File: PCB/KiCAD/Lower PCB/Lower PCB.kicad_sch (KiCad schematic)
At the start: 16 parts, among them J2 Conn_01x02, U1 ATmega328PB-A, Y1 Crystal

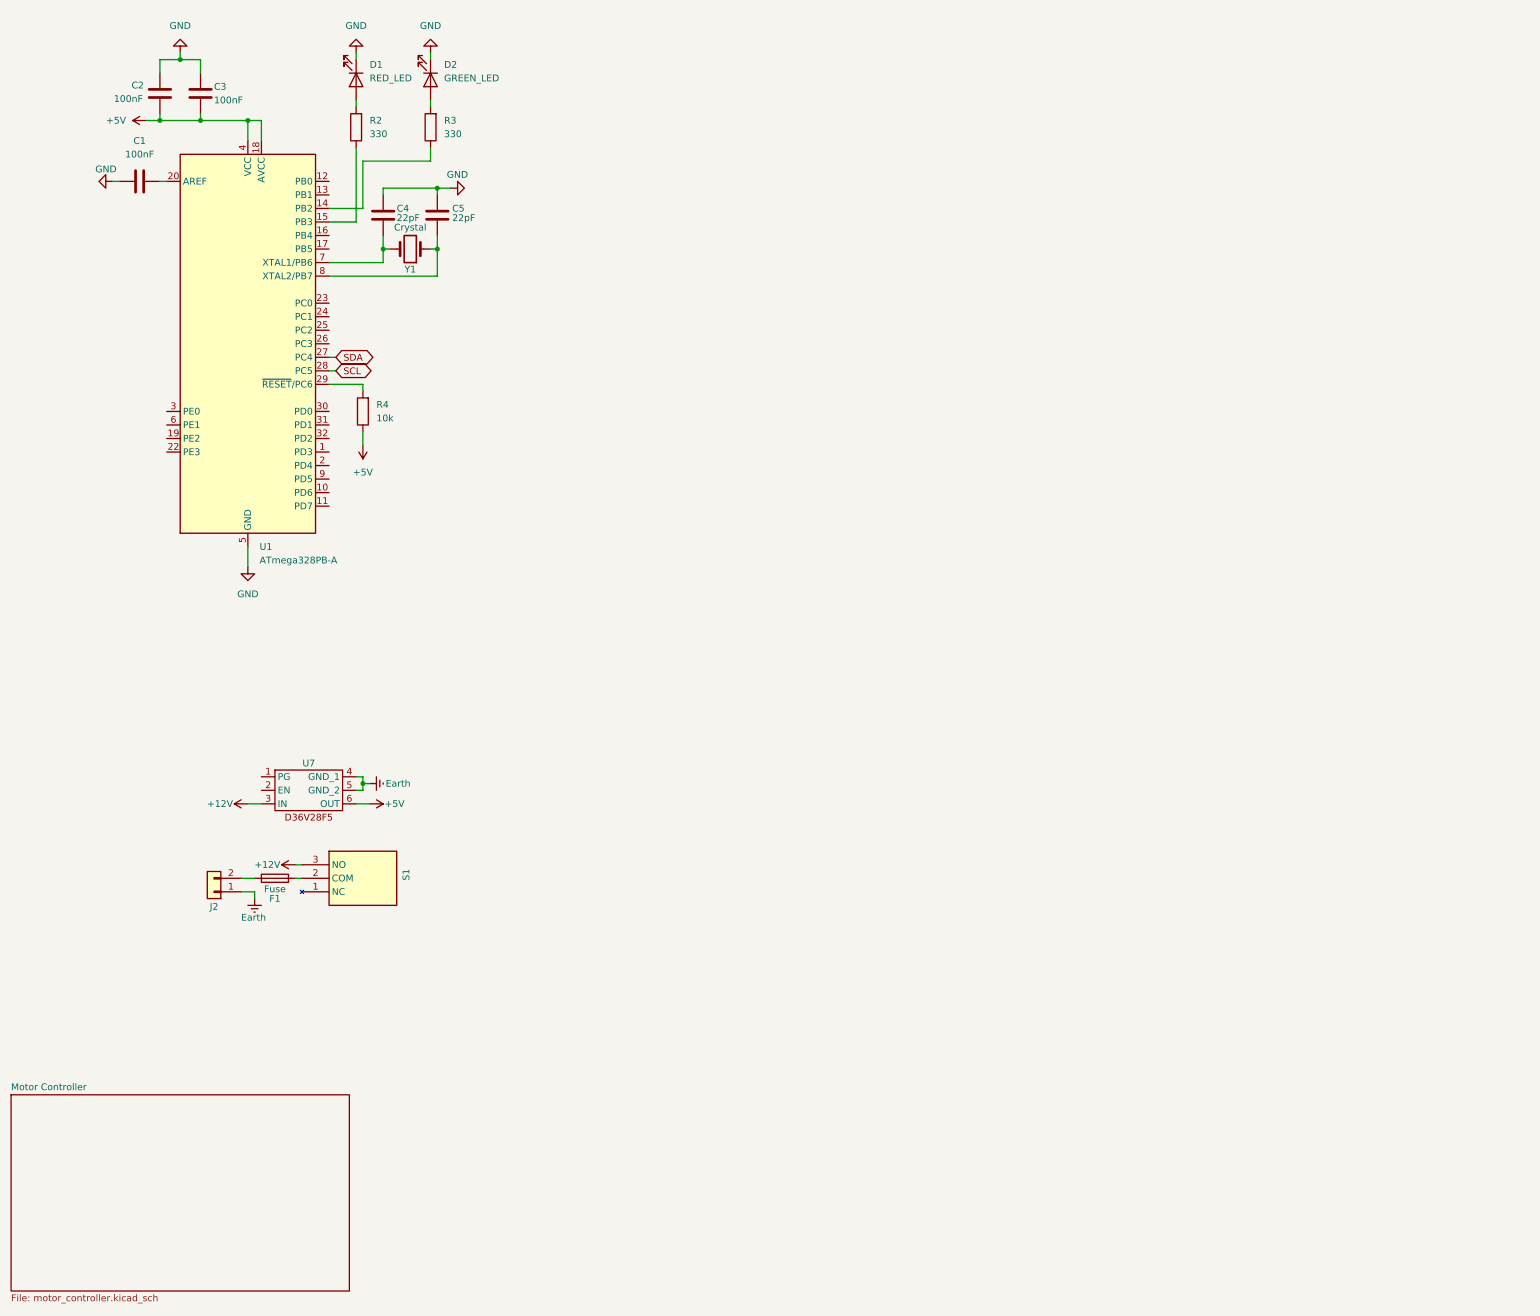
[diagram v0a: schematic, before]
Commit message: More work to the lower PCB
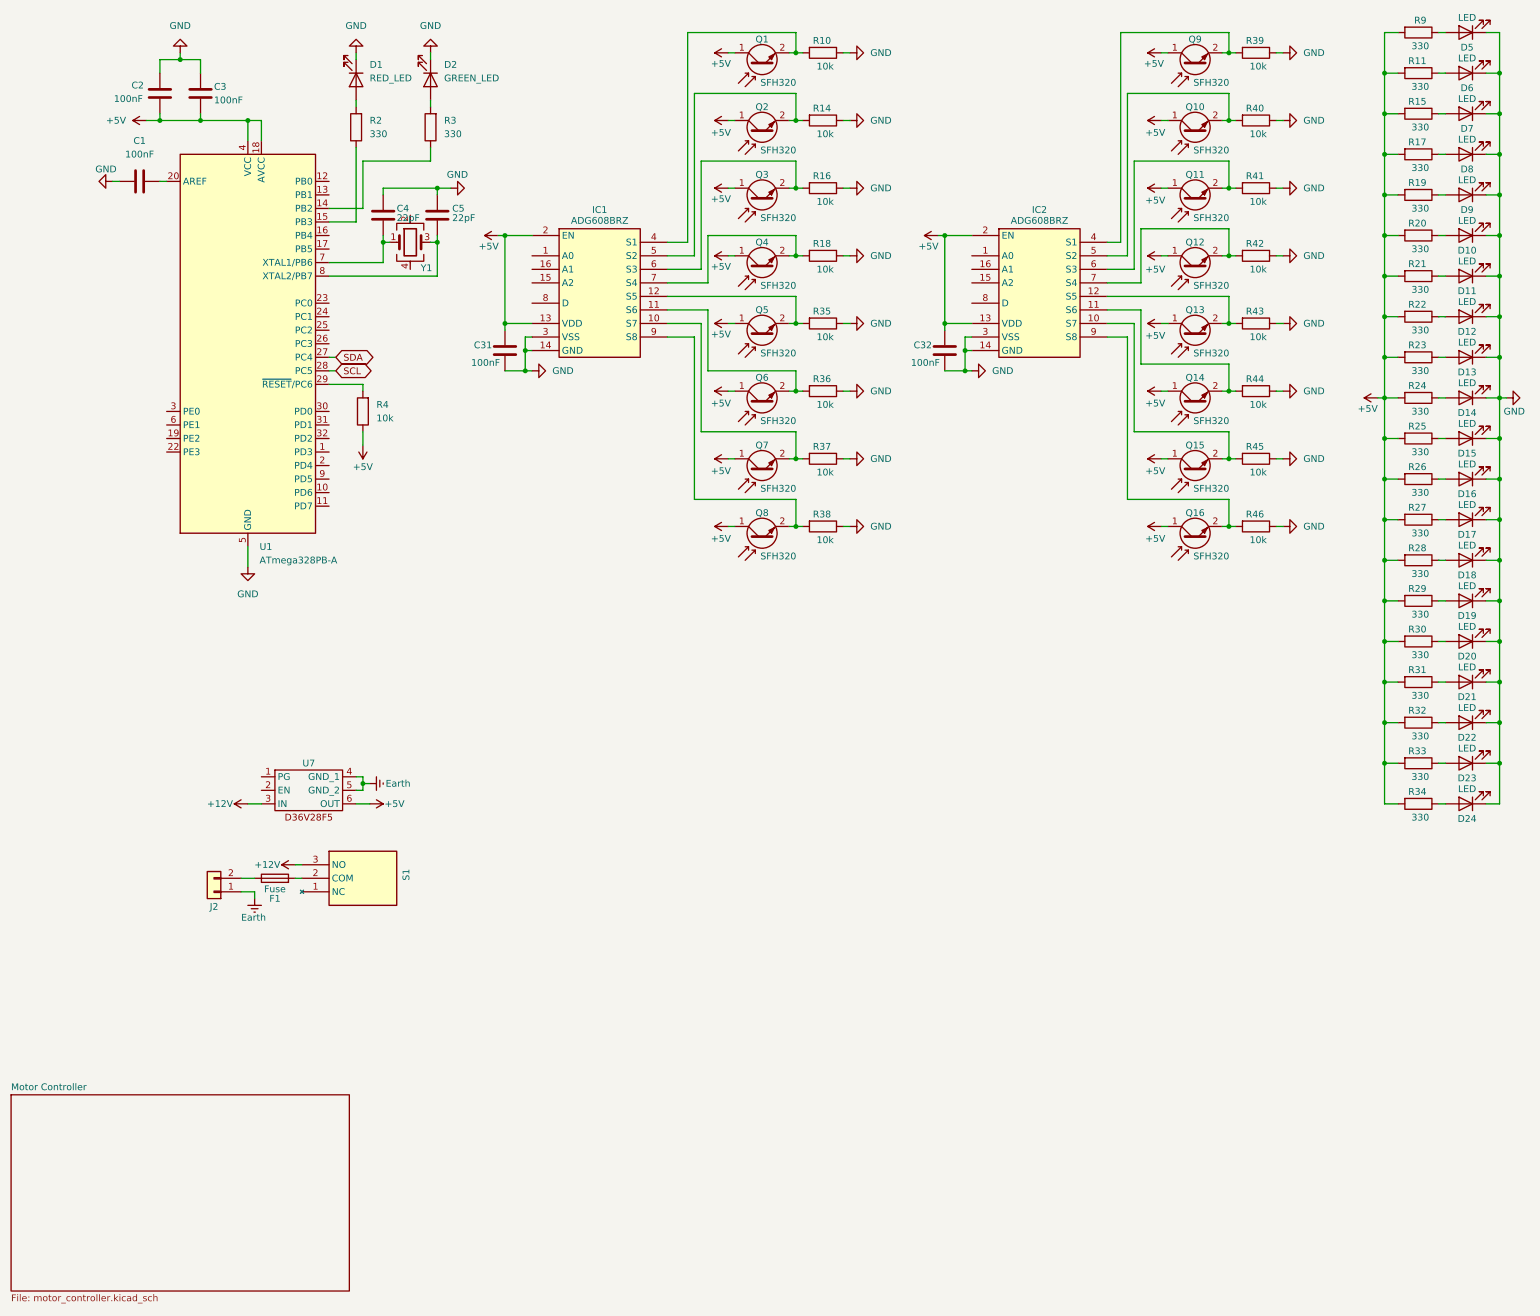
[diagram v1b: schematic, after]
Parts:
- removed Y1: Crystal, Crystal:Crystal_SMD_3225-4Pin_3.2x2.5mm_HandSoldering, symbol Device:Crystal
- added C31, C32: 100nF, Capacitor_SMD:C_0805_2012Metric_Pad1.18x1.45mm_HandSolder, symbol Device:C
- added D10, D11, D12, D13, D14, D15, D16, D17, D18, D19, D20, D21, D22, D23, D24, D5, D6, D7, D8, D9: LED, LED_SMD:LED_PLCC-2_3.4x3.0mm_KA, symbol Device:LED
- added IC1, IC2: ADG608BRZ, ADG608BRZ:SOIC127P600X175-16N, symbol ADG608BRZ:ADG608BRZ
- added Q1, Q10, Q11, Q12, Q13, Q14, Q15, Q16, Q2, Q3, Q4, Q5, Q6, Q7, Q8, Q9: SFH320, LED_SMD:LED_PLCC-2_3.4x3.0mm_KA, symbol Sensor_Optical:SFH320
- added R10, R14, R16, R18, R35, R36, R37, R38, R39, R40, R41, R42, R43, R44, R45, R46: 10k, Resistor_SMD:R_0805_2012Metric_Pad1.20x1.40mm_HandSolder, symbol Device:R
- added R11, R15, R17, R19, R20, R21, R22, R23, R24, R25, R26, R27, R28, R29, R30, R31, R32, R33, R34, R9: 330, Resistor_SMD:R_0805_2012Metric_Pad1.20x1.40mm_HandSolder, symbol Device:R
- added Y1: Crystal_GND24, Crystal:Crystal_SMD_5032-4Pin_5.0x3.2mm, symbol Device:Crystal_GND24
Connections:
- net +5V: now also C31.1, C32.1, IC1.13 (VDD), IC1.2 (EN), IC2.13 (VDD), IC2.2 (EN), Q1.1 (C), Q10.1 (C), Q11.1 (C), Q12.1 (C), Q13.1 (C), Q14.1 (C), Q15.1 (C), Q16.1 (C), Q2.1 (C), Q3.1 (C), Q4.1 (C), Q5.1 (C), Q6.1 (C), Q7.1 (C), Q8.1 (C), Q9.1 (C), R11.2, R15.2, R17.2, R19.2, R20.2, R21.2, R22.2, R23.2, R24.2, R25.2, R26.2, R27.2, R28.2, R29.2, R30.2, R31.2, R32.2, R33.2, R34.2, R9.2
- net GND: now also C31.2, C32.2, D10.1 (K), D11.1 (K), D12.1 (K), D13.1 (K), D14.1 (K), D15.1 (K), D16.1 (K), D17.1 (K), D18.1 (K), D19.1 (K), D20.1 (K), D21.1 (K), D22.1 (K), D23.1 (K), D24.1 (K), D5.1 (K), D6.1 (K), D7.1 (K), D8.1 (K), D9.1 (K), IC1.14 (GND), IC1.3 (VSS), IC2.14 (GND), IC2.3 (VSS), R10.1, R14.1, R16.1, R18.1, R35.1, R36.1, R37.1, R38.1, R39.1, R40.1, R41.1, R42.1, R43.1, R44.1, R45.1, R46.1
- net at C5.2, U1.8 (XTAL2/PB7): now also Y1.3
- net at C4.2, U1.7 (XTAL1/PB6): now also Y1.1
- new net: D7.2 (A), R15.1
- new net: IC1.4 (S1), Q1.2 (E), R10.2
- new net: D22.2 (A), R32.1
- new net: D23.2 (A), R33.1
- new net: D11.2 (A), R21.1
- new net: IC2.6 (S3), Q11.2 (E), R41.2
- new net: IC2.5 (S2), Q10.2 (E), R40.2
- new net: D19.2 (A), R29.1
- new net: D5.2 (A), R9.1
- new net: D14.2 (A), R24.1
- new net: IC1.5 (S2), Q2.2 (E), R14.2
- new net: D10.2 (A), R20.1
- new net: IC1.12 (S5), Q5.2 (E), R35.2
- new net: D13.2 (A), R23.1
- new net: IC2.7 (S4), Q12.2 (E), R42.2
- new net: IC2.11 (S6), Q14.2 (E), R44.2
- new net: IC1.9 (S8), Q8.2 (E), R38.2
- new net: D6.2 (A), R11.1
- new net: D9.2 (A), R19.1
- new net: D17.2 (A), R27.1
- new net: D21.2 (A), R31.1
- new net: D16.2 (A), R26.1
- new net: IC2.4 (S1), Q9.2 (E), R39.2
- new net: IC1.10 (S7), Q7.2 (E), R37.2
- new net: IC1.11 (S6), Q6.2 (E), R36.2
- new net: IC1.6 (S3), Q3.2 (E), R16.2
- new net: IC1.7 (S4), Q4.2 (E), R18.2
- new net: D8.2 (A), R17.1
- new net: D15.2 (A), R25.1
- new net: D12.2 (A), R22.1
- new net: D20.2 (A), R30.1
- new net: IC2.10 (S7), Q15.2 (E), R45.2
- new net: IC2.9 (S8), Q16.2 (E), R46.2
- new net: D24.2 (A), R34.1
- new net: D18.2 (A), R28.1
- new net: IC2.12 (S5), Q13.2 (E), R43.2
